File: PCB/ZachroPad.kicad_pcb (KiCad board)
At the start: 2 copper layers, 42.9 x 63 mm, 7 parts, among them SW1 SW_Push, SW2 SW_Push, SW3 SW_Push, SW4 SW_Push, U1 XIAO-RP2040-DIP

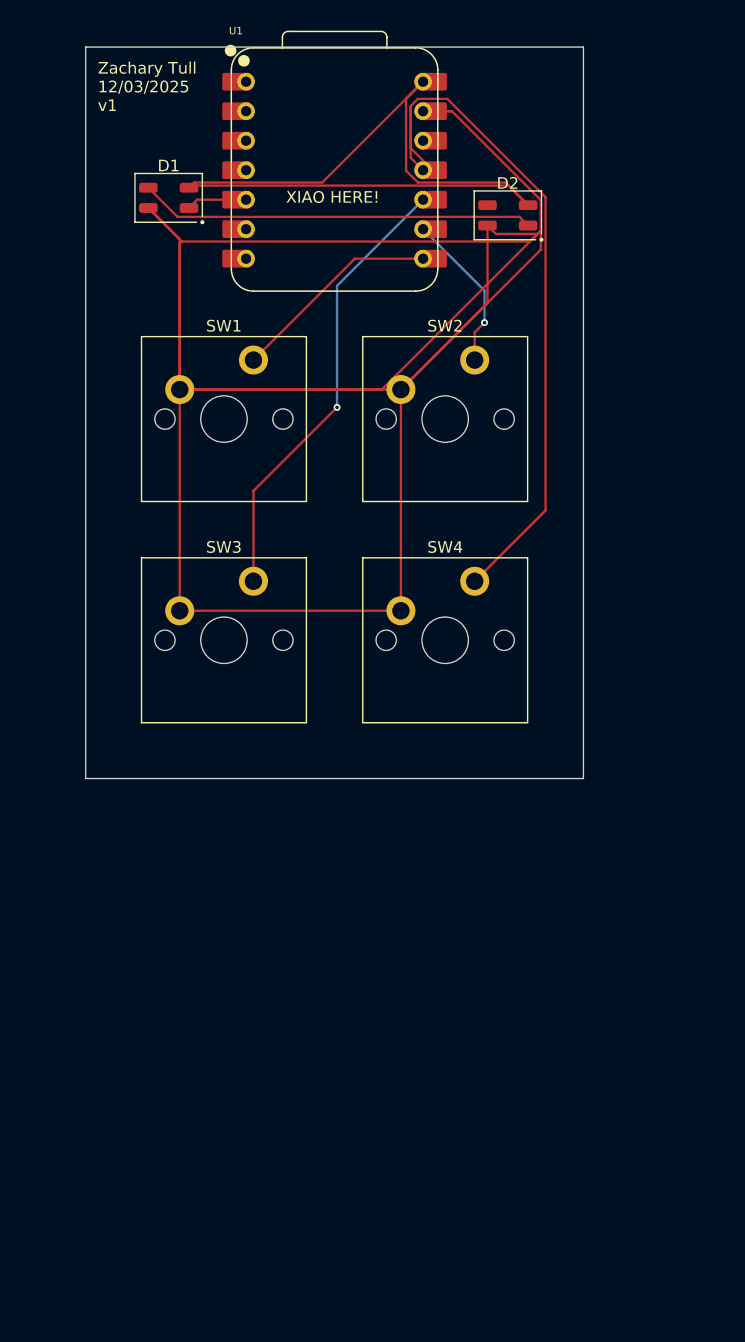
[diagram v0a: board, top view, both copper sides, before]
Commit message: updates!
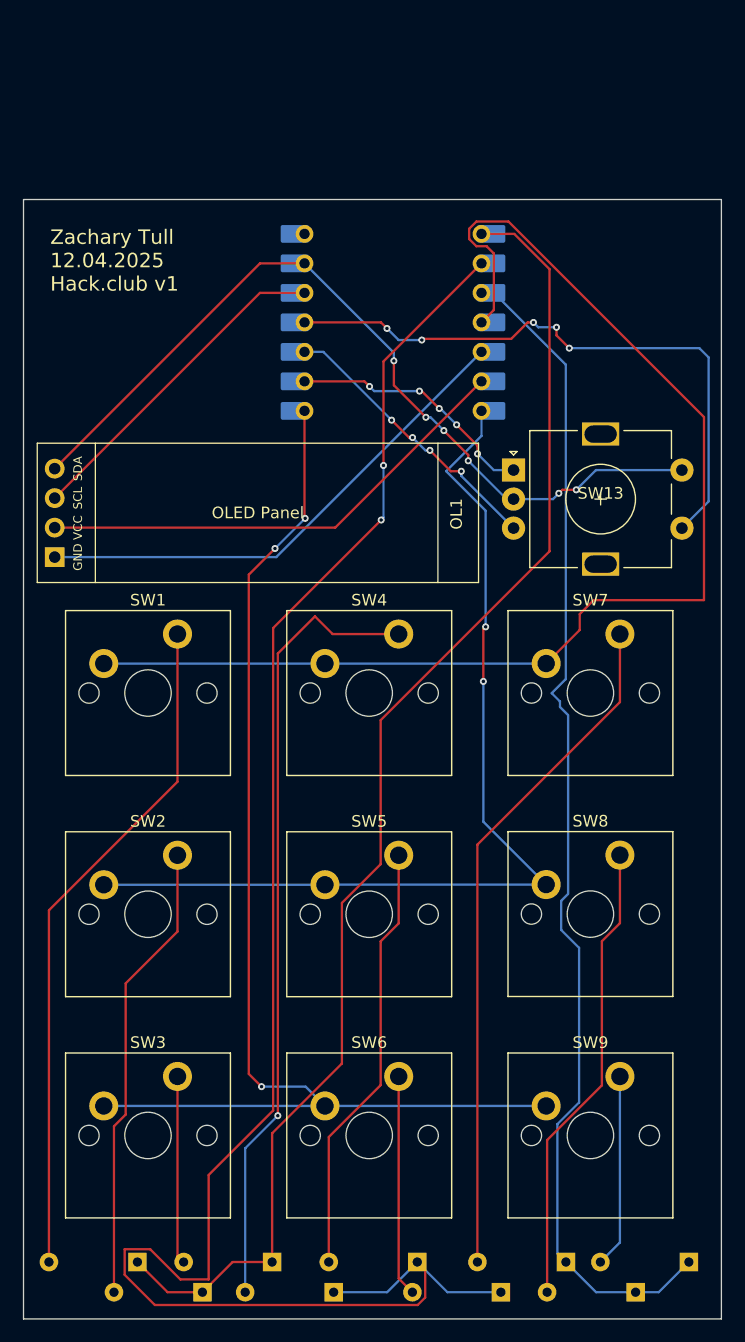
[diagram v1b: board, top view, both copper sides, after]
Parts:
- added D3: 1N4148, PCM_Diode_THT_AKL:D_DO-35_SOD27_P7.62mm_Horizontal, B.Cu at (123.2, 160.7)
- added D4: 1N4148, PCM_Diode_THT_AKL:D_DO-35_SOD27_P7.62mm_Horizontal, B.Cu at (128.5, 163.3)
- added D5: 1N4148, PCM_Diode_THT_AKL:D_DO-35_SOD27_P7.62mm_Horizontal, B.Cu at (135.7, 160.7)
- added D6: 1N4148, PCM_Diode_THT_AKL:D_DO-35_SOD27_P7.62mm_Horizontal, B.Cu at (142.9, 163.3)
- added D7: 1N4148, PCM_Diode_THT_AKL:D_DO-35_SOD27_P7.62mm_Horizontal, B.Cu at (148.5, 160.7)
- added D8: 1N4148, PCM_Diode_THT_AKL:D_DO-35_SOD27_P7.62mm_Horizontal, B.Cu at (154.5, 163.3)
- added D9: 1N4148, PCM_Diode_THT_AKL:D_DO-35_SOD27_P7.62mm_Horizontal, B.Cu at (159.1, 160.7)
- added OL1: OLED, OLED:SSD1306-0.91-OLED-4pin-128x32, F.Cu at (141.0, 102.2)
- added SW13: RotaryEncoder_Switch, Rotary Encoder:RotaryEncoder_Alps_EC11E-Switch_Vertical_H20mm, F.Cu at (144.0, 92.5)
- added SW5: SW_Push, PCM_Switch_Keyboard_Cherry_MX:SW_Cherry_MX_PCB_1.00u, F.Cu at (131.6, 130.8)
- added SW6: SW_Push, PCM_Switch_Keyboard_Cherry_MX:SW_Cherry_MX_PCB_1.00u, F.Cu at (131.6, 149.8)
- added SW7: SW_Push, PCM_Switch_Keyboard_Cherry_MX:SW_Cherry_MX_PCB_1.00u, F.Cu at (150.6, 111.7)
- added SW8: SW_Push, PCM_Switch_Keyboard_Cherry_MX:SW_Cherry_MX_PCB_1.00u, F.Cu at (150.6, 130.7)
- added SW9: SW_Push, PCM_Switch_Keyboard_Cherry_MX:SW_Cherry_MX_PCB_1.00u, F.Cu at (150.6, 149.8)
- D1, D2: value SK6812MINI -> 1N4148; footprint PCM_LED_SMD_AKL:LED_SK6812MINI_PLCC4_3.5x3.5mm_P1.75mm -> PCM_Diode_THT_AKL:D_DO-35_SOD27_P7.62mm_Horizontal; moved to B.Cu
- U1: moved to B.Cu
- moved D2 96.4 mm to (117.2, 163.3), turned to 180 degrees
- moved D1 91.7 mm to (111.6, 160.7), turned to 180 degrees
- moved SW2 49.7 mm to (112.5, 130.8)
- moved SW3 43.1 mm to (112.5, 149.8)
- moved SW1 24.5 mm to (112.5, 111.7)
- moved U1 14.0 mm to (133.6, 79.8), turned to 180 degrees
- moved SW4 7.97 mm to (131.6, 111.7)
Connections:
- D1 pad 1: Net-(D1-DOUT) -> Net-(D1-K)
- D1 pad 2: GND -> Net-(D1-A)
- D2 pad 1: unconnected-(D2-DOUT-Pad1) -> Net-(D1-K)
- D2 pad 2: GND -> Net-(D2-A)
- SW1 pad 1: GND -> Net-(U1-GPIO29/ADC3/A3)
- SW1 pad 2: Net-(U1-GPIO1/RX) -> Net-(D1-A)
- SW2 pad 1: GND -> Net-(U1-GPIO0/TX)
- SW2 pad 2: Net-(U1-GPIO2/SCK) -> Net-(D2-A)
- SW3 pad 1: GND -> Net-(U1-GPIO1/RX)
- SW3 pad 2: Net-(U1-GPIO4/MISO) -> Net-(D3-A)
- SW4 pad 1: GND -> Net-(U1-GPIO29/ADC3/A3)
- SW4 pad 2: Net-(U1-GPIO3/MOSI) -> Net-(D4-A)
- U1 pad 1: unconnected-(U1-GPIO26/ADC0/A0-Pad1) -> Net-(D1-K)
- U1 pad 12: unconnected-(U1-3V3-Pad12) -> +3V3
- U1 pad 14: +5V -> unconnected-(U1-VBUS-Pad14)
- U1 pad 2: unconnected-(U1-GPIO27/ADC1/A1-Pad2) -> Net-(D4-K)
- U1 pad 3: unconnected-(U1-GPIO28/ADC2/A2-Pad3) -> Net-(D7-K)
- U1 pad 4: unconnected-(U1-GPIO29/ADC3/A3-Pad4) -> Net-(U1-GPIO29/ADC3/A3)
- U1 pad 5: Net-(D1-DIN) -> Net-(OL1-SDA)
- U1 pad 6: unconnected-(U1-GPIO7/SCL-Pad6) -> Net-(OL1-SCL)
- U1 pad 7: unconnected-(U1-GPIO0/TX-Pad7) -> Net-(U1-GPIO0/TX)
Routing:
- net GND: track 239.1 -> 72.7 mm, vias 0 -> 6
- net Net-(D4-K): track 0.00 -> 154.9 mm, vias 0 -> 2
- net Net-(D1-K): track 0.00 -> 116.3 mm
- net Net-(U1-GPIO29/ADC3/A3): track 0.00 -> 107.9 mm
- net Net-(D7-K): track 0.00 -> 102.9 mm
- net Net-(U1-GPIO1/RX): track 18.2 -> 104.9 mm, vias 0 -> 3
- net Net-(U1-GPIO0/TX): track 0.00 -> 83.9 mm, vias 0 -> 2
- net +5V: track 73.9 -> 0.00 mm
- net Net-(D4-A): track 0.00 -> 68.5 mm, vias 0 -> 1
- net Net-(D7-A): track 0.00 -> 59.2 mm
- net Net-(D1-A): track 0.00 -> 58.7 mm
- net Net-(OL1-SDA): track 0.00 -> 44.1 mm
- net Net-(OL1-SCL): track 0.00 -> 42.0 mm
- net Net-(D8-A): track 0.00 -> 40.2 mm
- net Net-(D2-A): track 0.00 -> 39.9 mm
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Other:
- board size 42.9 x 63 mm -> 60.1 x 96.4 mm
- board text added: "Zachary Tull 12.04.2025 Hack.club v1"
- board text removed: "Zachary Tull 12/03/2025 v1"
